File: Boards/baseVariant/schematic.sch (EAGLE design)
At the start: 109 parts, among them IC1 LM2596S, J1 MAX9850ETI+, Q1 BSS84, Q2 BSS84, Q3 BSS84, Q4 BSS84, Q5 BSS84

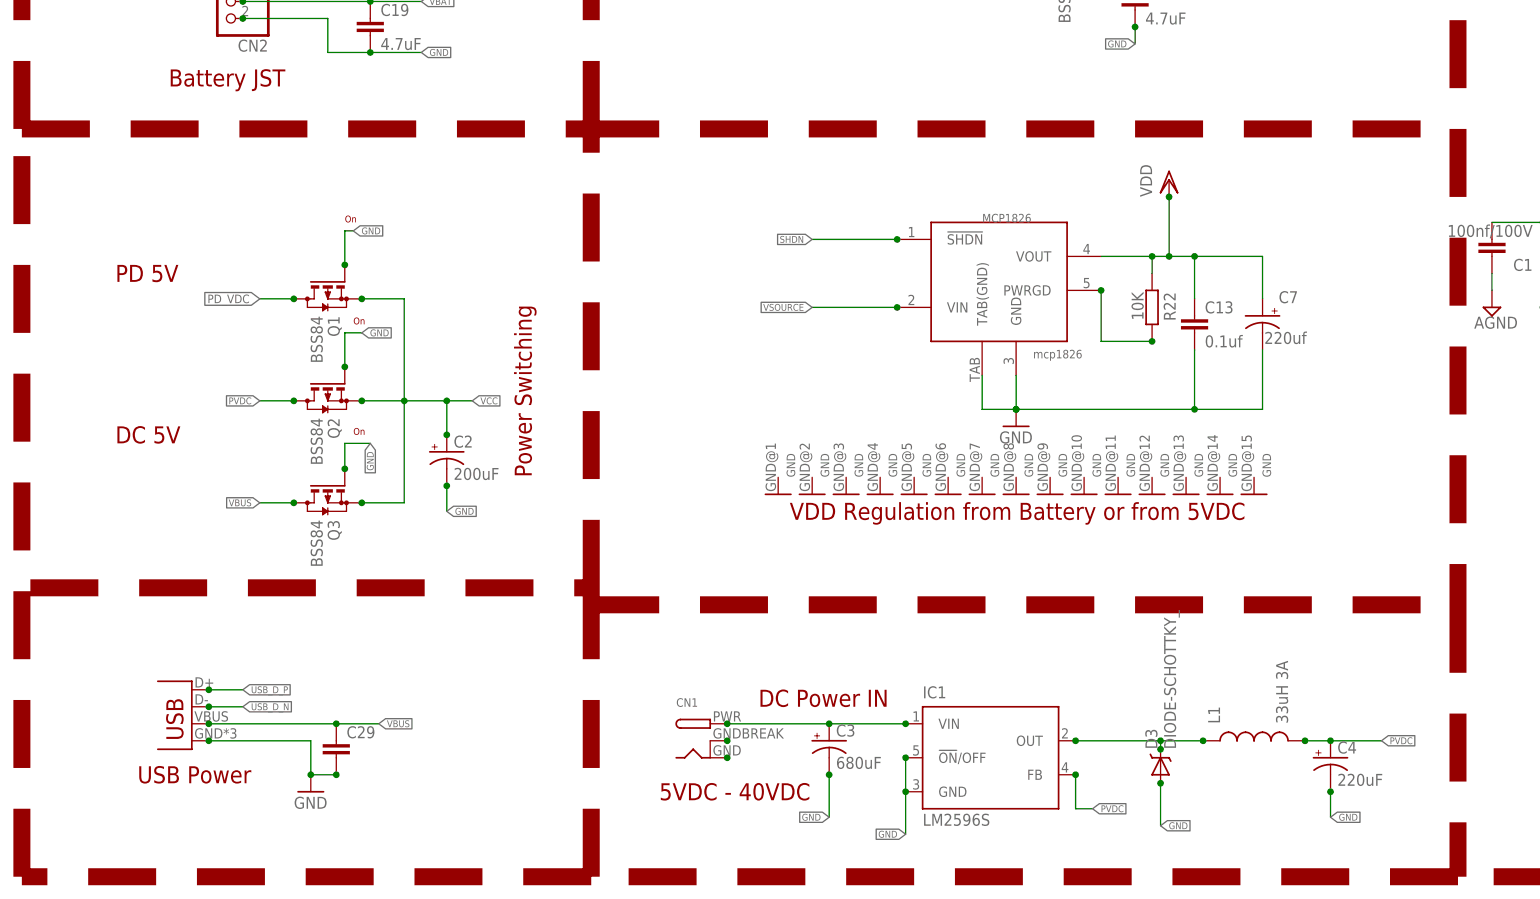
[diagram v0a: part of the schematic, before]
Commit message: Normal Push
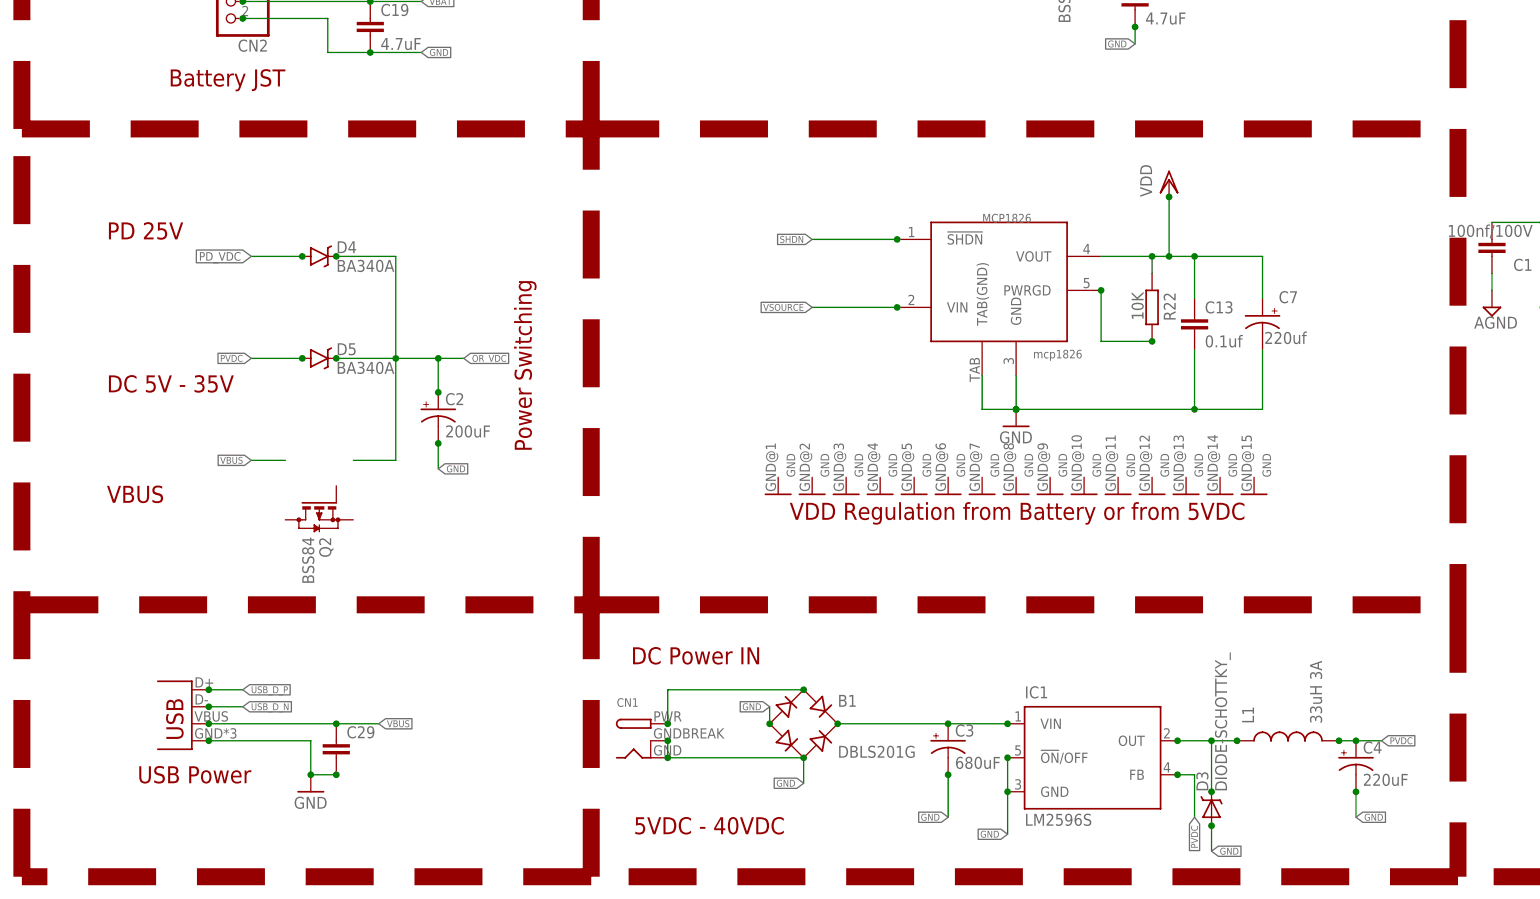
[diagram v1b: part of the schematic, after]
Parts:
- removed Q1, Q3: BSS84, transistor-small-signal:BSS84
- added B1: DBLS201G, rectifier:DBLS201G
- added D4, D5: BA340A, SparkFun-DiscreteSemi:B340A
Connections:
- removed net N$14: CN1.GND
- removed net N$30: C3.+, CN1.PWR, IC1.VIN
- removed net N$5: CN1.GNDBREAK
- new net N$17: B1.AC1, CN1.PWR
- new net N$31: B1.+, C3.+, IC1.VIN
- new net OR_VDC: C2.+, D4.C, D5.C
- net GND: now also B1.-, B1.AC2, CN1.GND, CN1.GNDBREAK; no longer Q1.G, Q2.G, Q3.G
- net PD_VDC: now also D4.A; no longer Q1.D
- net PVDC: now also D5.A; no longer Q2.D
- net VBUS: no longer Q3.D
- net VCC: no longer C2.+, Q1.S, Q2.S, Q3.S
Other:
- note added: "DC 5V - 35V"
- note added: "PD 25V"
- note added: "VBUS"
- note removed: "DC 5V"
- note removed: "On"
- note removed: "PD 5V"
- moved on the sheet: C2, C3, C4, CN1, D3, IC1, L1, Q2
